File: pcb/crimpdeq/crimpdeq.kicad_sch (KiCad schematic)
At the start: 55 parts, among them J10 A-_Cable_Pad, J11 E+_Cable_Pad, J12 E-_Cable_Pad, J2 USB4105-GF-A, J5 B-_Cable_Pad, J6 SW+_Cable_Pad, J7 B+_Cable_Pad, J8 SW-_Cable_Pad, J9 A+_Cable_Pad, Q2 DMG3415U, U1 ESP32-C3-MINI-1, U2 MCP73831T-2ACI/OT, U3 ADS1220, U5 MAX17048G+T10, U6 SY8088

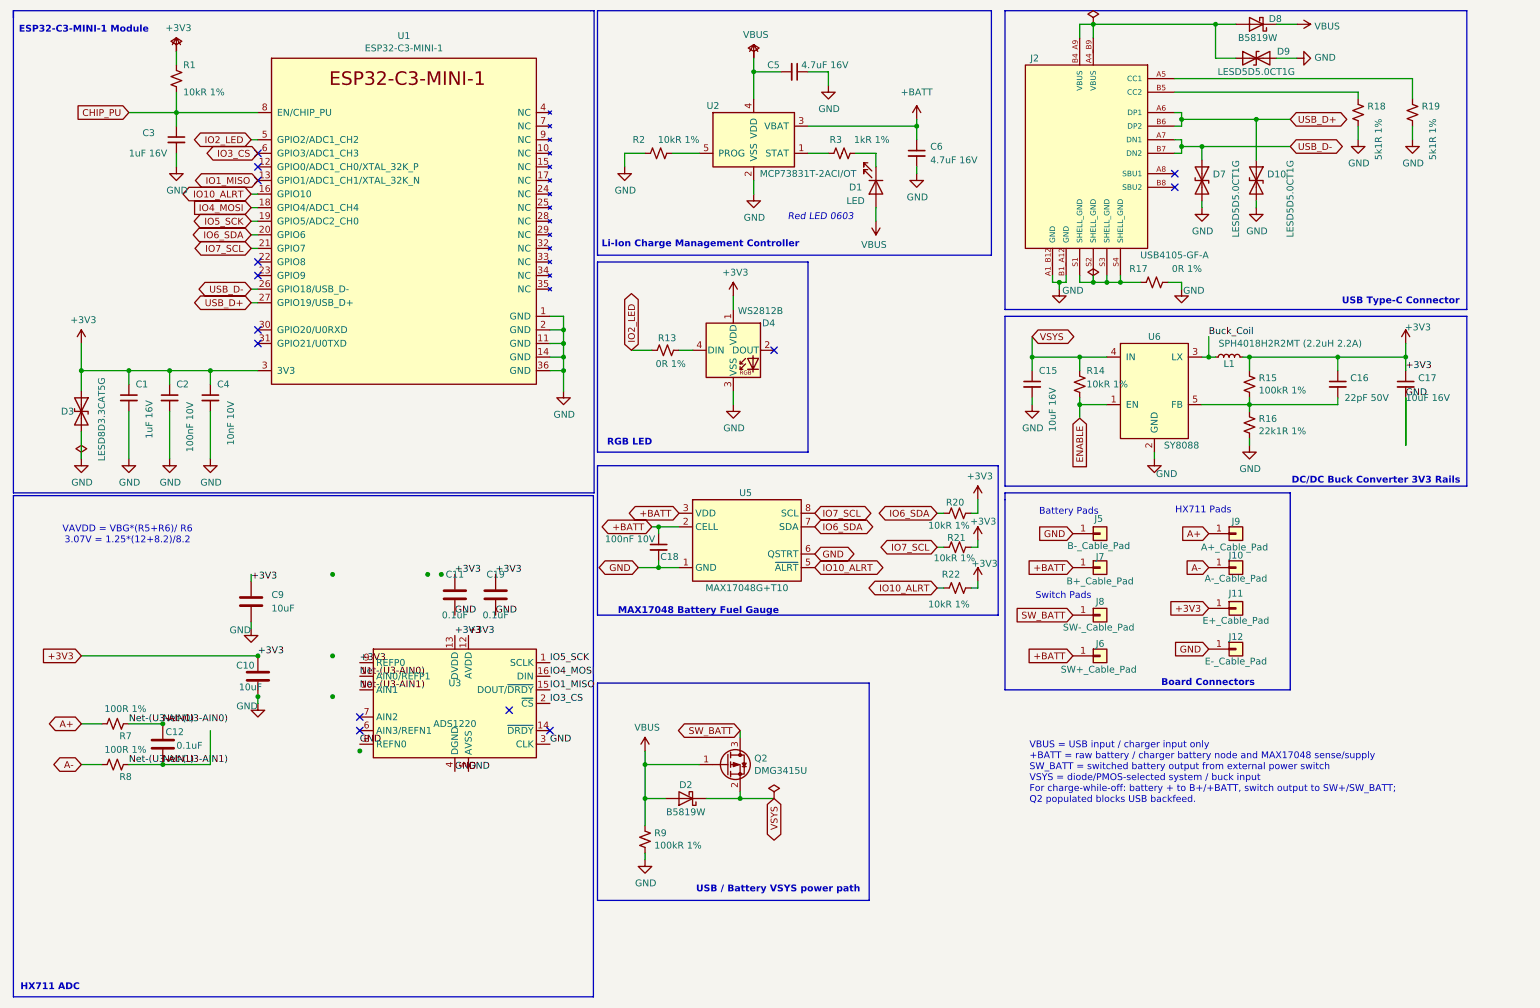
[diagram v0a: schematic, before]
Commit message: fix: clean up schematic connections
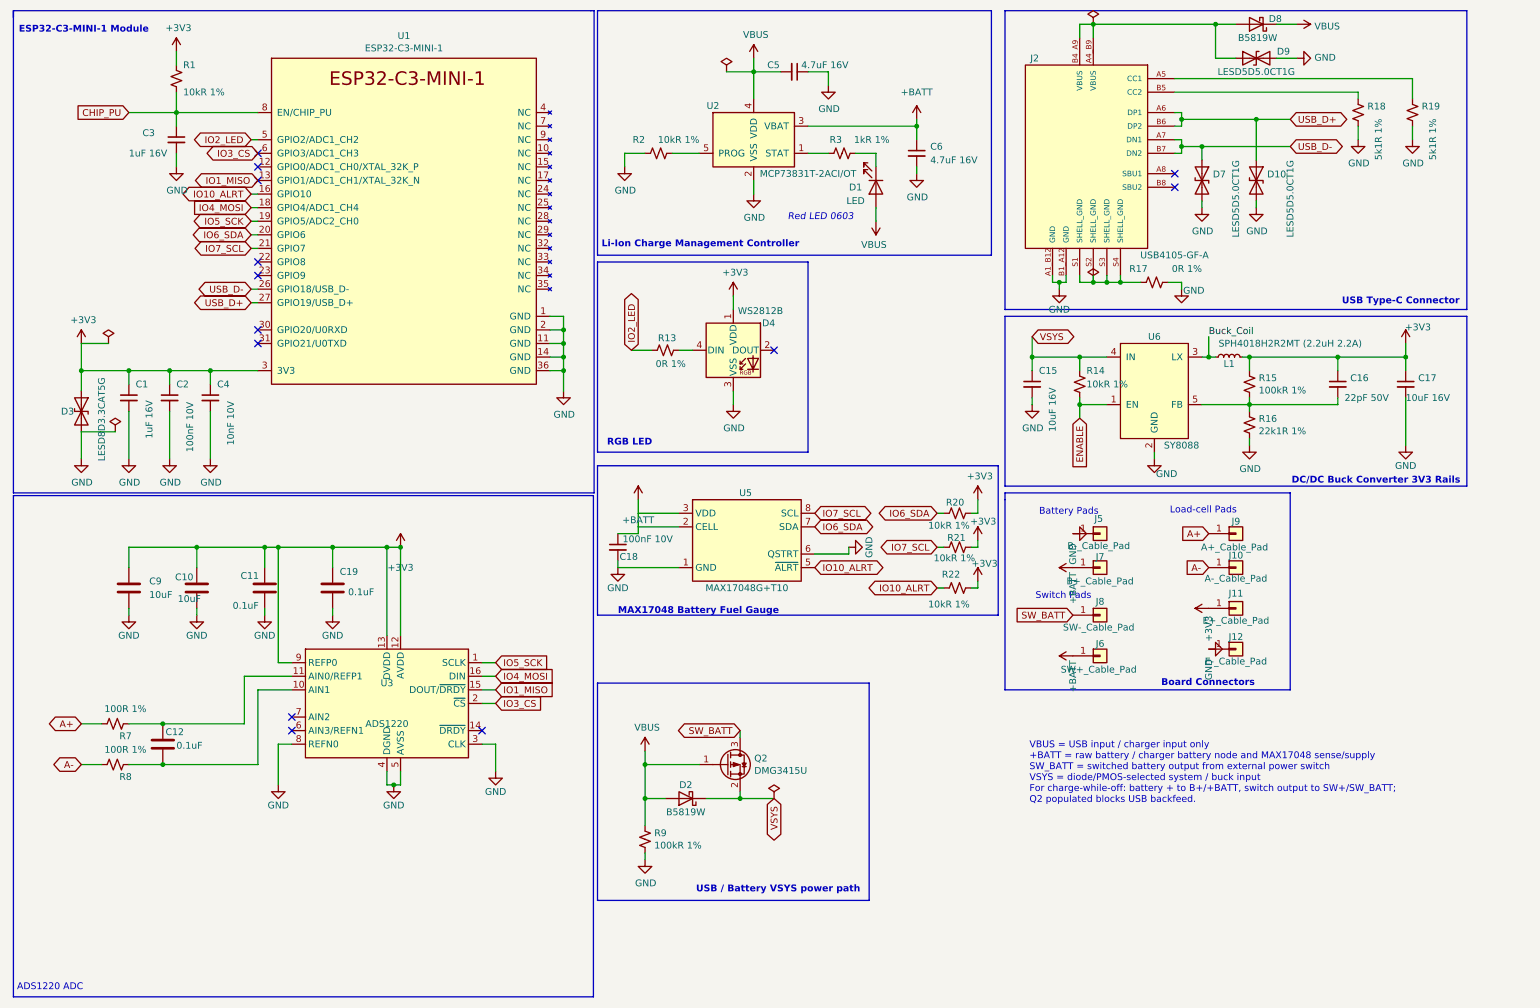
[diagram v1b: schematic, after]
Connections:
- net Net-(U3-AIN0): no longer names the net of C12.1, R7.1, U3.11 (AIN0/REFP1)
- net Net-(U3-AIN1): no longer names the net of C12.2, R8.1, U3.10 (AIN1)
- no-connect marks 14 -> 13
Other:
- note added: "ADS1220 ADC"
- note added: "Load-cell Pads"
- note removed: "HX711 ADC"
- note removed: "HX711 Pads"
- note removed: "VAVDD = VBG*(R5+R6)/ R6 3.07V = 1.25*(12+8.2)/8.2"
- moved on the sheet: C10, C18, C9
